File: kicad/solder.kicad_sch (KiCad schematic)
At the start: 10 parts, among them SW1 SW_Push, SW3 SW_Push, SW5 SW_Push

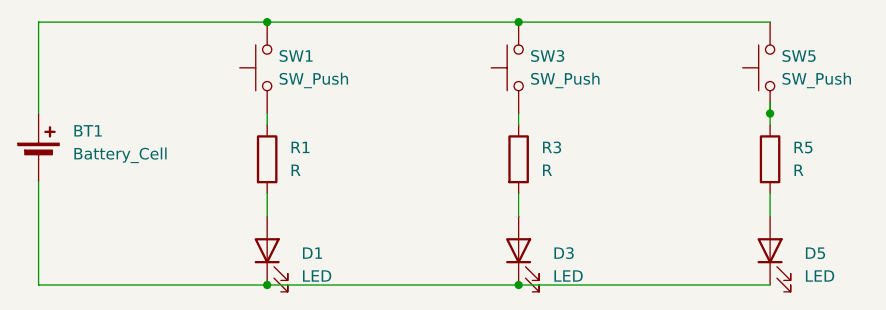
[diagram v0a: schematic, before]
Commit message: update pcb
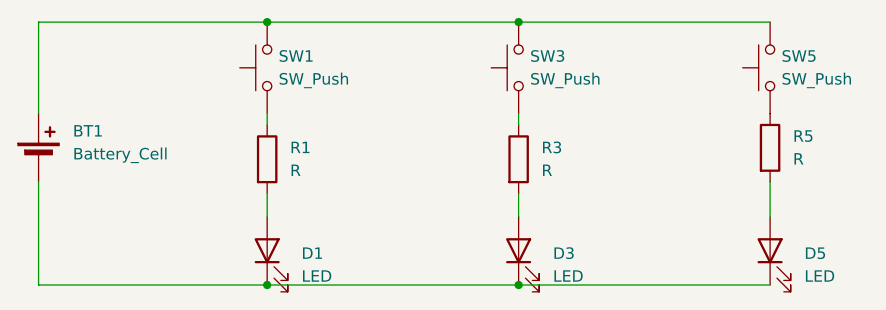
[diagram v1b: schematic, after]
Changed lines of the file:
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@@
 		(color 0 0 0 0)
 	)
-	(junction
-		(at 148.59 68.58)
-		(diameter 0)
-		(color 0 0 0 0)
-	)
 	(wire
 		(pts
@@
 	(wire
 		(pts
+			(xy 148.59 76.2) (xy 148.59 80.01)
+		)
+		(stroke
+			(width 0)
+			(type default)
+		)
+	)
+	(wire
+		(pts
 			(xy 120.65 58.42) (xy 92.71 58.42)
 		)
@@
 	(wire
 		(pts
-			(xy 148.59 77.47) (xy 148.59 80.01)
-		)
-		(stroke
-			(width 0)
-			(type default)
-		)
-	)
-	(wire
-		(pts
 			(xy 67.31 58.42) (xy 67.31 68.58)
 		)
@@
 	(wire
 		(pts
-			(xy 148.59 68.58) (xy 148.59 67.31)
-		)
-		(stroke
-			(width 0)
-			(type default)
-		)
-	)
-	(wire
-		(pts
 			(xy 92.71 58.42) (xy 67.31 58.42)
-		)
-		(stroke
-			(width 0)
-			(type default)
-		)
-	)
-	(wire
-		(pts
-			(xy 148.59 68.58) (xy 148.59 69.85)
 		)
 		(stroke
@@
 	)
 	(symbol
-		(lib_id "Device:R")
-		(at 148.59 73.66 0)
-		(unit 1)
-		(exclude_from_sim no)
-		(in_bom yes)
-		(on_board yes)
-		(dnp no)
-		(fields_autoplaced yes)
-		(property "Reference" "R5"
-			(at 151.13 72.3899 0)
-			(effects
-				(font
-					(size 1.27 1.27)
-				)
-				(justify left)
-			)
-		)
-		(property "Value" "R"
-			(at 151.13 74.9299 0)
-			(effects
-				(font
-					(size 1.27 1.27)
-				)
-				(justify left)
-			)
-		)
-		(property "Footprint" "Resistor_THT:R_Axial_DIN0207_L6.3mm_D2.5mm_P7.62mm_Horizontal"
-			(at 146.812 73.66 90)
-			(effects
-				(font
-					(size 1.27 1.27)
-				)
-				(hide yes)
-			)
-		)
-		(property "Datasheet" "~"
-			(at 148.59 73.66 0)
-			(effects
-				(font
-					(size 1.27 1.27)
-				)
-				(hide yes)
-			)
-		)
-		(property "Description" "Resistor"
-			(at 148.59 73.66 0)
-			(effects
-				(font
-					(size 1.27 1.27)
-				)
-				(hide yes)
-			)
-		)
-		(pin "1"
-		)
-		(pin "2"
-		)
-		(instances
-			(project "solder"
-				(path "/6b1a3850-b159-4b8c-9c15-11a3f2b97aa2"
-					(reference "R5")
-					(unit 1)
-				)
-			)
-		)
-	)
-	(symbol
 		(lib_id "Switch:SW_Push")
 		(at 92.71 63.5 90)
@@
 					(unit 1)
 				)
+			)
+		)
+	)
+	(symbol
+		(lib_id "Device:R")
+		(at 148.59 72.39 0)
+		(unit 1)
+		(exclude_from_sim no)
+		(in_bom yes)
+		(on_board yes)
+		(dnp no)
+		(fields_autoplaced yes)
+		(property "Reference" "R5"
+			(at 151.13 71.1199 0)
+			(effects
+				(font
+					(size 1.27 1.27)
+				)
+				(justify left)
+			)
+		)
+		(property "Value" "R"
+			(at 151.13 73.6599 0)
+			(effects
+				(font
+					(size 1.27 1.27)
+				)
+				(justify left)
+			)
+		)
+		(property "Footprint" "Resistor_THT:R_Axial_DIN0207_L6.3mm_D2.5mm_P7.62mm_Horizontal"
+			(at 146.812 72.39 90)
+			(effects
+				(font
+					(size 1.27 1.27)
+				)
+				(hide yes)
+			)
+		)
+		(property "Datasheet" "~"
+			(at 148.59 72.39 0)
+			(effects
+				(font
+					(size 1.27 1.27)
+				)
+				(hide yes)
+			)
+		)
+		(property "Description" "Resistor"
+			(at 148.59 72.39 0)
+			(effects
+				(font
+					(size 1.27 1.27)
+				)
+				(hide yes)
+			)
+		)
+		(pin "1"
+		)
+		(pin "2"
+		)
+		(instances
+			(project "solder"
+				(path "/6b1a3850-b159-4b8c-9c15-11a3f2b97aa2"
+					(reference "R5")
+					(unit 1)
+				)
